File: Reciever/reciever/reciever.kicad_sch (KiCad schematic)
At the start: 22 parts, among them J1 USB_C_Receptacle_USB2.0_14P, J2 UART/I2C, J3 TWAI, SW1 Button, SW2 Button, U1 TXS0102DCU, U2 LM66200, U3 SE5218ALG-LF, U4 ESP32-C6-MINI-1, U5 TCAN330DR

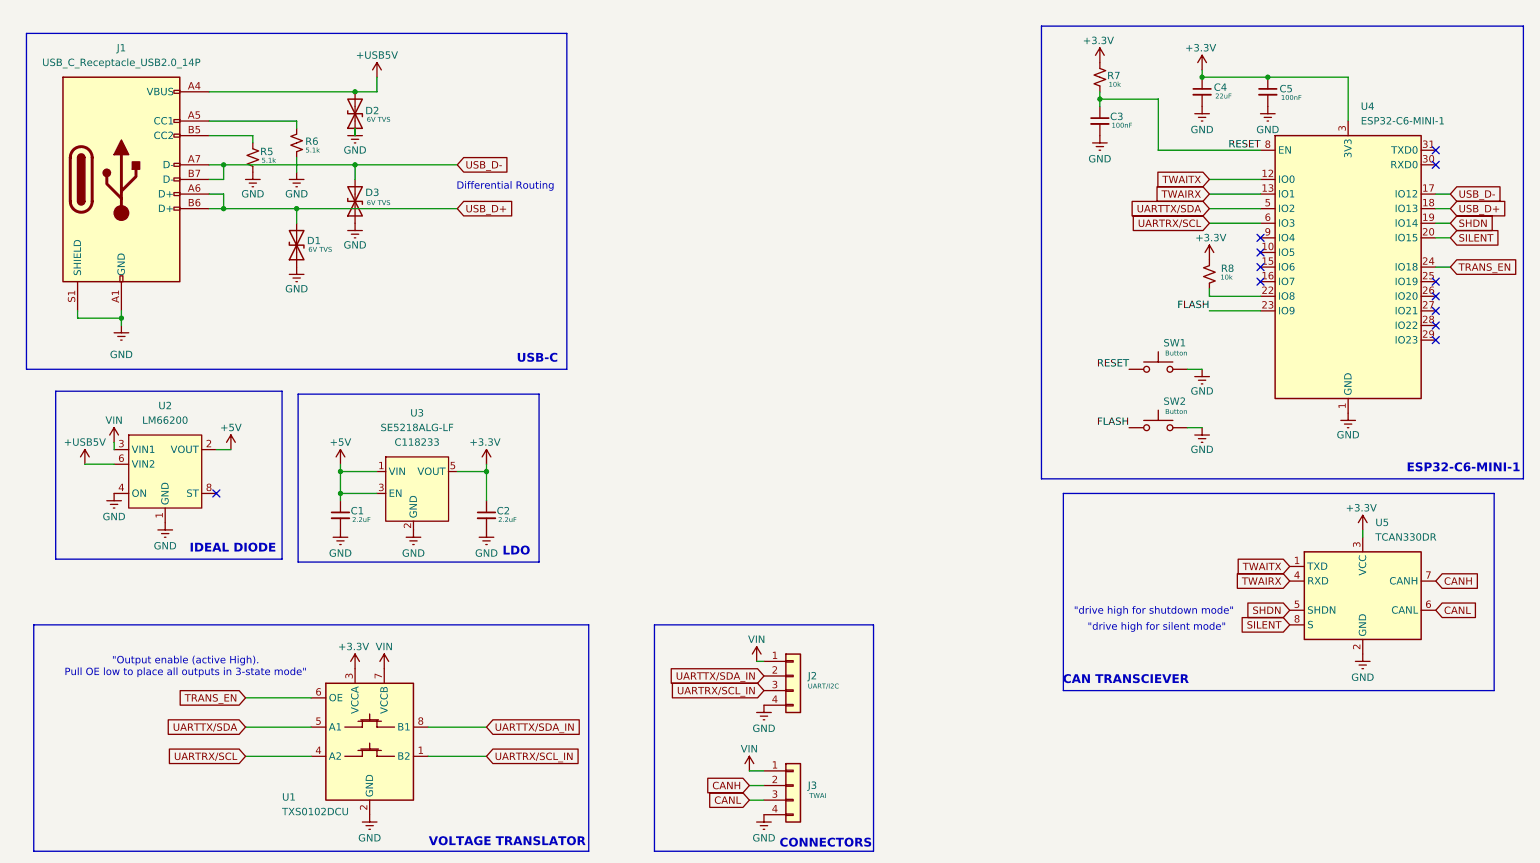
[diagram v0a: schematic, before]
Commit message: crc v2
finalizing receiver layout
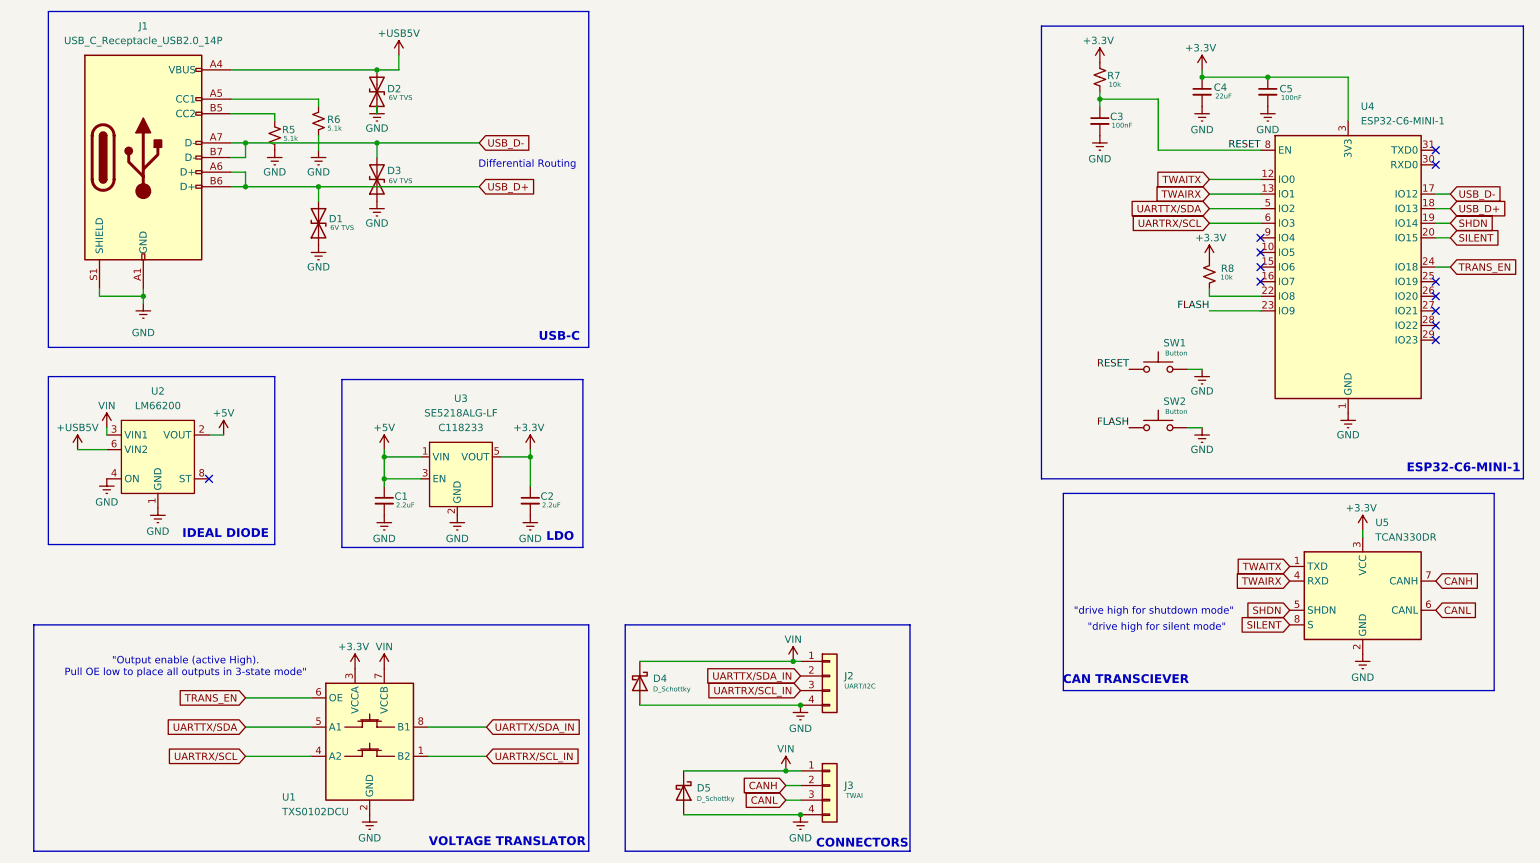
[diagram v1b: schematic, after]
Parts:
- added D4, D5: D_Schottky, Diode_SMD:D_SOD-123, symbol Device:D_Schottky
- U2: LCSC# (none) -> C3235556
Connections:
- net GND: now also D4.2 (A), D5.2 (A)
- net VIN: now also D4.1 (K), D5.1 (K)
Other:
- moved on the sheet: C1, C2, D1, D2, D3, J1, J2, J3, R5, R6, U2, U3
